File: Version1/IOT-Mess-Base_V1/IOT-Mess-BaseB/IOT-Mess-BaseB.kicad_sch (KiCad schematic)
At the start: 18 parts, among them J1 Milk-V Duo, J2 SuperMini_ESP32-H2, J3 CH_P20, J4 Lolin32-Lite, J5 Conn_01x04_Pin, J6 Conn_01x38_Pin, J7 Conn_01x20_Pin, J8 Conn_01x03_Pin, J9 Conn_01x11_Pin, Q5 AO3400A, SW3 SW_Push

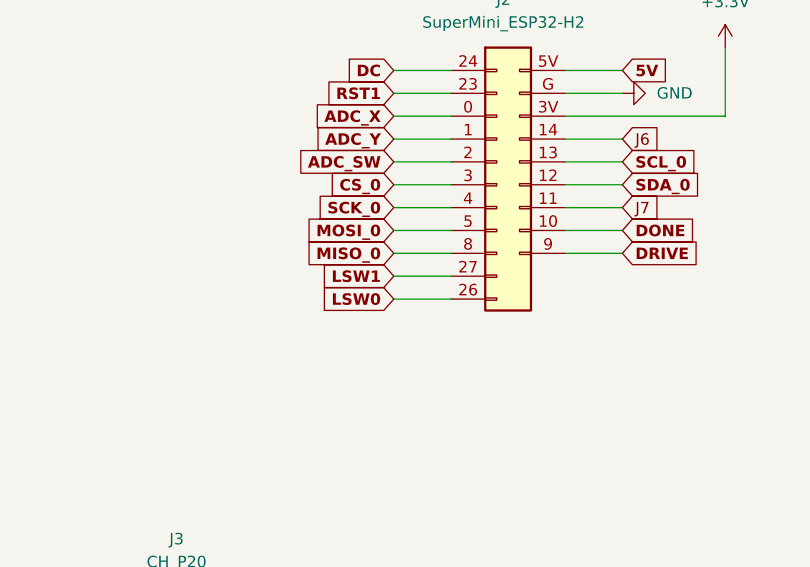
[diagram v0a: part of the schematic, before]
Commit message: added jumper boards.
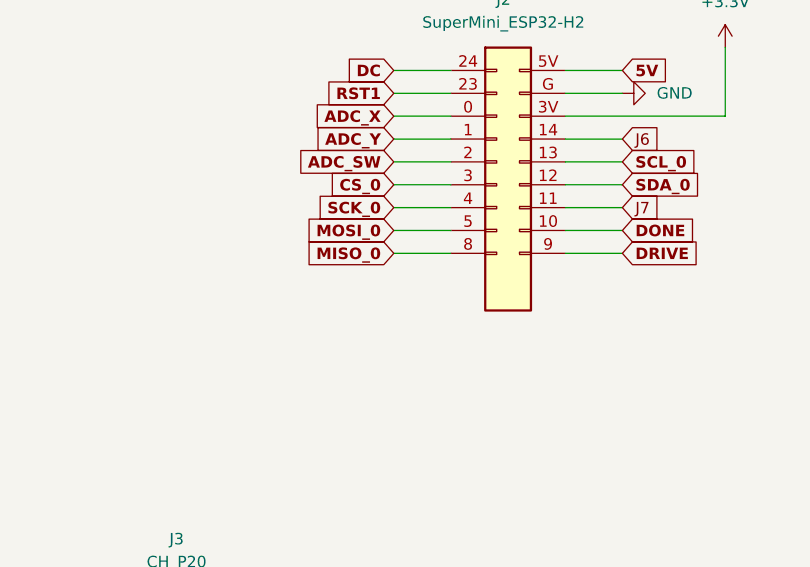
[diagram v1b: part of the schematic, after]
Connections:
- net LSW0: no longer J2.26 (Pin_2)
- net LSW1: no longer J2.27 (Pin_1)
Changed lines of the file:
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@@
 				)
 				(rectangle
-					(start -1.27 -12.573)
-					(end 0 -12.827)
-					(stroke
-						(width 0.1524)
-						(type default)
-					)
-					(fill
-						(type none)
-					)
-				)
-				(rectangle
-					(start -1.27 -15.113)
-					(end 0 -15.367)
-					(stroke
-						(width 0.1524)
-						(type default)
-					)
-					(fill
-						(type none)
-					)
-				)
-				(rectangle
 					(start 3.81 10.287)
 					(end 2.54 10.033)
@@
 				)
 				(pin passive line
-					(at -5.08 -12.7 0)
-					(length 3.81)
-					(name "Pin_1"
-						(effects
-							(font
-								(size 1.27 1.27)
-							)
-						)
-					)
-					(number "27"
-						(effects
-							(font
-								(size 1.27 1.27)
-							)
-						)
-					)
-				)
-				(pin passive line
-					(at -5.08 -15.24 0)
-					(length 3.81)
-					(name "Pin_2"
-						(effects
-							(font
-								(size 1.27 1.27)
-							)
-						)
-					)
-					(number "26"
-						(effects
-							(font
-								(size 1.27 1.27)
-							)
-						)
-					)
-				)
-				(pin passive line
 					(at 7.62 10.16 180)
 					(length 3.81)
@@
 	(wire
 		(pts
-			(xy 118.11 81.28) (xy 111.76 81.28)
-		)
-		(stroke
-			(width 0)
-			(type default)
-		)
-	)
-	(wire
-		(pts
 			(xy 344.17 96.52) (xy 344.17 102.87)
 		)
@@
 	(wire
 		(pts
-			(xy 118.11 78.74) (xy 111.76 78.74)
-		)
-		(stroke
-			(width 0)
-			(type default)
-		)
-	)
-	(wire
-		(pts
 			(xy 344.17 91.44) (xy 344.17 96.52)
 		)
@@
 		)
 	)
-	(global_label "LSW1"
-		(shape input)
-		(at 111.76 78.74 180)
-		(fields_autoplaced yes)
-		(effects
-			(font
-				(size 1.27 1.27)
-				(thickness 0.254)
-				(bold yes)
-				(color 0 0 255 1)
-			)
-			(justify right)
-		)
-		(property "Intersheetrefs" "${INTERSHEET_REFS}"
-			(at 103.4003 78.74 0)
-			(effects
-				(font
-					(size 1.27 1.27)
-				)
-				(justify right)
-				(hide yes)
-			)
-		)
-	)
 	(global_label "SDA_0"
 		(shape input)
@@
 		)
 	)
-	(global_label "LSW0"
-		(shape input)
-		(at 111.76 81.28 180)
-		(fields_autoplaced yes)
-		(effects
-			(font
-				(size 1.27 1.27)
-				(thickness 0.254)
-				(bold yes)
-				(color 0 0 255 1)
-			)
-			(justify right)
-		)
-		(property "Intersheetrefs" "${INTERSHEET_REFS}"
-			(at 103.8763 81.28 0)
-			(effects
-				(font
-					(size 1.27 1.27)
-				)
-				(justify right)
-				(hide yes)
-			)
-		)
-	)
 	(global_label "SDA_0"
 		(shape input)
@@
 		(pin "2"
 		)
-		(pin "27"
-		)
-		(pin "26"
-		)
 		(instances
